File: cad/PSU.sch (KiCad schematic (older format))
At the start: 16 parts, among them J1 Input, J2 Barrel_Jack_Switch, J3 Output, J4 INA219 breakout, J5 WWG-A, J6 WWG-B, Q1 LM317T, U1 LM7805_TO220, U2 X9C103P

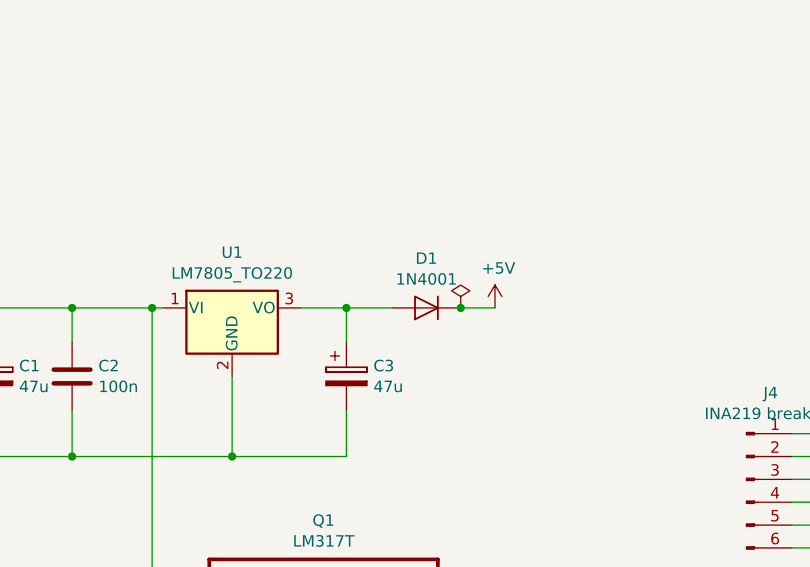
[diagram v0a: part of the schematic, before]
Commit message: layout again
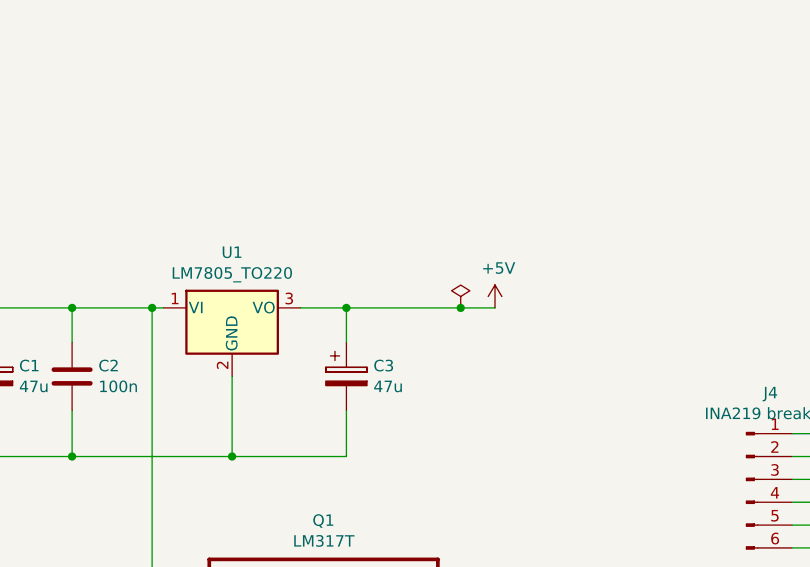
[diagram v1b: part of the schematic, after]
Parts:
- removed D1: 1N4001, Diode_THT:D_DO-41_SOD81_P10.16mm_Horizontal, symbol Diode:1N4001
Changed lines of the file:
@@
 	7150 3200 7200 3200
-Wire Wire Line
-	3900 2650 4100 2650
 Wire Wire Line
 	4400 2650 4550 2650
@@
 NoConn ~ 7200 3500
 NoConn ~ 5000 5050
-$Comp
-L Diode:1N4001 D1
-U 1 1 5CE7B69A
-P 4250 2650
-F 0 "D1" H 4250 2434 50  0000 C CNN
-F 1 "1N4001" H 4250 2525 50  0000 C CNN
-F 2 "Diode_THT:D_DO-41_SOD81_P10.16mm_Horizontal" H 4250 2475 50  0001 C CNN
-F 3 "http://www.vishay.com/docs/88503/1n4001.pdf" H 4250 2650 50  0001 C CNN
-	1    4250 2650
-	-1   0    0    1
-$EndComp
-Connection ~ 4400 2650
 Wire Wire Line
 	5500 4000 5700 4000
@@
 Wire Wire Line
 	6050 3600 7200 3600
+Wire Wire Line
+	3900 2650 4400 2650
+Connection ~ 4400 2650
 $EndSCHEMATC
